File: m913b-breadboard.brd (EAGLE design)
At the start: 17.8 x 44.4 mm, 14 parts

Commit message: Add missing female connectors
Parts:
- added U1, U2: IDC 2x5 FEMALE, hardware:EMPTY
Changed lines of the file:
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@@
 <element name="HL2" library="optoelectronics" package="LED2X5" value="BLUE(2MMX5MM)" x="7.62" y="1.905" smashed="yes" rot="R180"/>
 <element name="PCB1" library="module-footprints" package="EMPTY" value="M913b rev.A" x="0" y="0"/>
+<element name="U1" library="hardware" package="EMPTY" value="IDC 2x5 FEMALE" x="-1.016" y="0"/>
+<element name="U2" library="hardware" package="EMPTY" value="IDC 2x5 FEMALE" x="-2.032" y="0"/>
 </elements>
 <signals>

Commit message: Misc. component update
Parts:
- U1, U2: value IDC 2x5 FEMALE -> IDC 2x5 CABLE
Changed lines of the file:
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@@
 <element name="HL2" library="optoelectronics" package="LED2X5" value="BLUE(2MMX5MM)" x="7.62" y="1.905" smashed="yes" rot="R180"/>
 <element name="PCB1" library="module-footprints" package="EMPTY" value="M913b rev.A" x="0" y="0"/>
-<element name="U1" library="hardware" package="EMPTY" value="IDC 2x5 FEMALE" x="-1.016" y="0"/>
-<element name="U2" library="hardware" package="EMPTY" value="IDC 2x5 FEMALE" x="-2.032" y="0"/>
+<element name="U1" library="hardware" package="EMPTY" value="IDC 2x5 CABLE" x="-1.016" y="0"/>
+<element name="U2" library="hardware" package="EMPTY" value="IDC 2x5 CABLE" x="-2.032" y="0"/>
 </elements>
 <signals>

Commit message: Add ERM1-4MM for LEDs
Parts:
- added U3, U4: ERM1-4MM, hardware:EMPTY
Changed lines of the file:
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@@
 <element name="U1" library="hardware" package="EMPTY" value="IDC 2x5 CABLE" x="-1.016" y="0"/>
 <element name="U2" library="hardware" package="EMPTY" value="IDC 2x5 CABLE" x="-2.032" y="0"/>
+<element name="U3" library="hardware" package="EMPTY" value="ERM1-4MM" x="-3" y="-1.25">
+<attribute name="MOUSER" value="749-ERM1-4MM" x="-3" y="-1.25" size="1.778" layer="27" display="off"/>
+</element>
+<element name="U4" library="hardware" package="EMPTY" value="ERM1-4MM" x="-4" y="-2.5">
+<attribute name="MOUSER" value="749-ERM1-4MM" x="-4" y="-2.5" size="1.778" layer="27" display="off"/>
+</element>
 </elements>
 <signals>

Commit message: M913 Component Values Update
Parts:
- removed U3, U4: ERM1-4MM, hardware:EMPTY
- C1, C2: value 10U/35V(11MM) -> 10U/35V
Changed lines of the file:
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@@
 </autorouter>
 <elements>
-<element name="C1" library="capacitors-electrolytic" package="E2-5" value="10U/35V(11MM)" x="7.62" y="37.06" rot="R270">
-<attribute name="MOUSER" value="75-515D106M035JA6AE3" x="7.62" y="37.06" size="1.778" layer="27" rot="R270" display="off"/>
+<element name="C1" library="capacitors-electrolytic" package="E2-5" value="10U/35V" x="7.62" y="37.06" rot="R270">
+<attribute name="MOUSER" value="647-USW1V100MDD" x="7.62" y="37.06" size="1.778" layer="27" rot="R270" display="off"/>
 </element>
-<element name="C2" library="capacitors-electrolytic" package="E2-5" value="10U/35V(11MM)" x="7.62" y="7.39" rot="R270">
-<attribute name="MOUSER" value="75-515D106M035JA6AE3" x="7.62" y="7.39" size="1.778" layer="27" rot="R270" display="off"/>
+<element name="C2" library="capacitors-electrolytic" package="E2-5" value="10U/35V" x="7.62" y="7.39" rot="R270">
+<attribute name="MOUSER" value="647-USW1V100MDD" x="7.62" y="7.39" size="1.778" layer="27" rot="R270" display="off"/>
 </element>
 <element name="R1" library="resistors" package="R-0207/10" value="10R(TH)" x="1.27" y="38.1" rot="R90">
@@
 <element name="U1" library="hardware" package="EMPTY" value="IDC 2x5 CABLE" x="-1.016" y="0"/>
 <element name="U2" library="hardware" package="EMPTY" value="IDC 2x5 CABLE" x="-2.032" y="0"/>
-<element name="U3" library="hardware" package="EMPTY" value="ERM1-4MM" x="-3" y="-1.25">
-<attribute name="MOUSER" value="749-ERM1-4MM" x="-3" y="-1.25" size="1.778" layer="27" display="off"/>
-</element>
-<element name="U4" library="hardware" package="EMPTY" value="ERM1-4MM" x="-4" y="-2.5">
-<attribute name="MOUSER" value="749-ERM1-4MM" x="-4" y="-2.5" size="1.778" layer="27" display="off"/>
-</element>
 </elements>
 <signals>

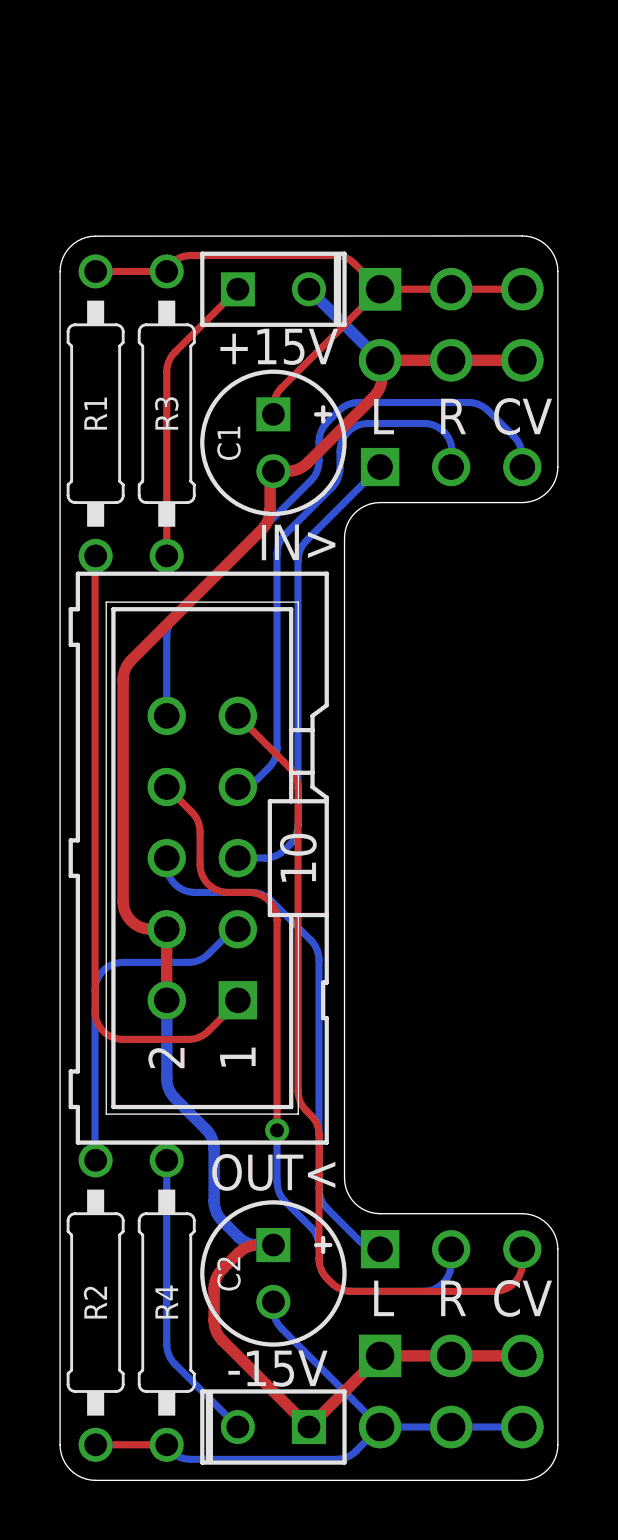
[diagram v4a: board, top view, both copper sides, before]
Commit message: Fix M913b Board
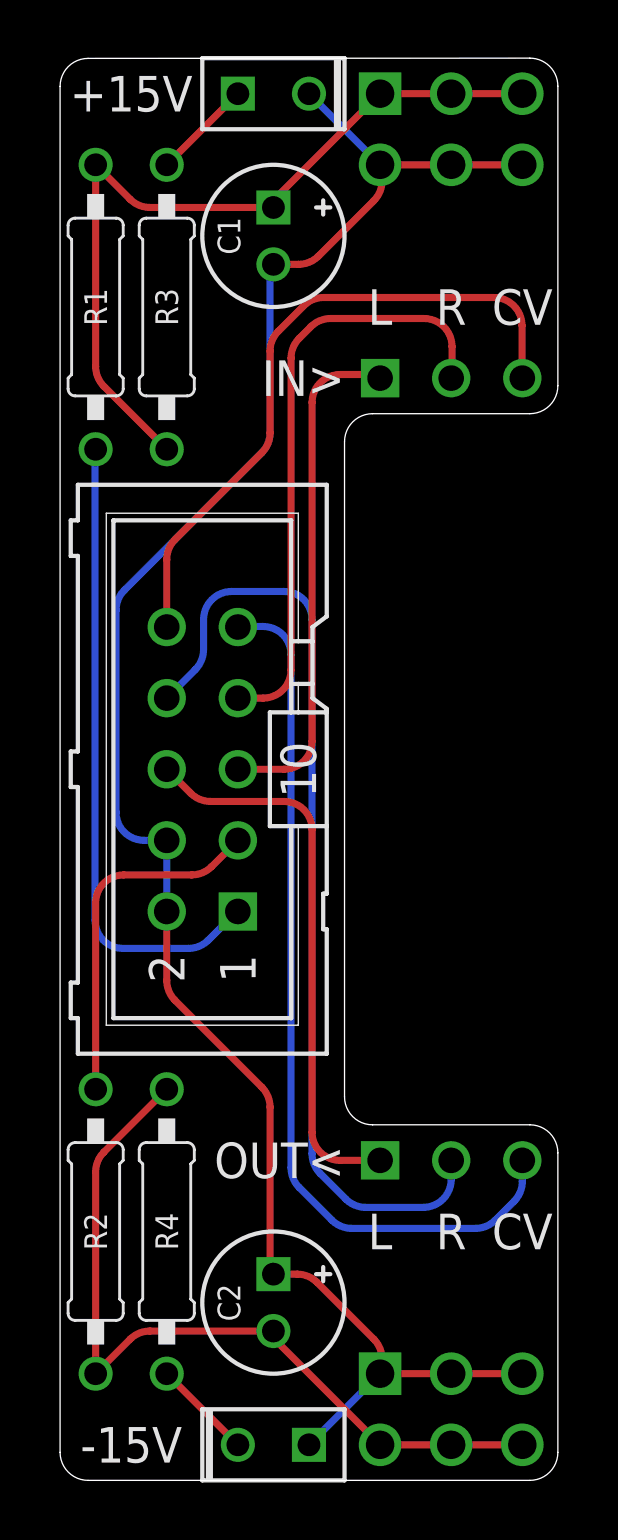
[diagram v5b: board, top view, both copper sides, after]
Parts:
- moved C1 7.39 mm to (7.62, 44.5)
- moved HL1 6.98 mm to (7.62, 49.5)
- moved XP4 6.98 mm to (14.0, 48.3)
- moved R1 3.81 mm to (1.27, 41.9)
- moved R3 3.81 mm to (3.81, 41.9), turned to 90 degrees
- moved XP3 3.17 mm to (11.4, 11.4)
- moved XP1 3.17 mm to (5.08, 25.4)
- moved XP2 3.17 mm to (11.4, 39.4)
- moved R2 2.54 mm to (1.27, 8.89)
- moved R4 2.54 mm to (3.81, 8.89), turned to 270 degrees
- moved C2 1.04 mm to (7.62, 6.35)
- moved HL2 0.64 mm to (7.62, 1.27)
- moved XP5 0.63 mm to (14.0, 2.54)
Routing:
- net N$9: track 25.6 -> 34.1 mm, vias 1 -> 0
- net N$4: track 10.5 -> 3.59 mm
- net N$1: track 10.5 -> 3.59 mm
- net +15V: track 21.9 -> 28.8 mm
- net -15V: track 22.0 -> 28.8 mm
- net GND: track 65.1 -> 69.9 mm
- net N$6: track 18.9 -> 21.5 mm
- net N$10: track 29.2 -> 31.5 mm
- net N$7: track 21.2 -> 23.5 mm
- net N$5: track 16.7 -> 18.1 mm
- net N$8: track 18.6 -> 19.7 mm
- net N$3: track 12.0 -> 12.6 mm
- net N$2: track 22.3 -> 22.8 mm
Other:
- board size 17.8 x 44.4 mm -> 17.8 x 50.8 mm
